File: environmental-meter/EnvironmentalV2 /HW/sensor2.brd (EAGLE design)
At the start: 66.7 x 50.6 mm, 16 parts

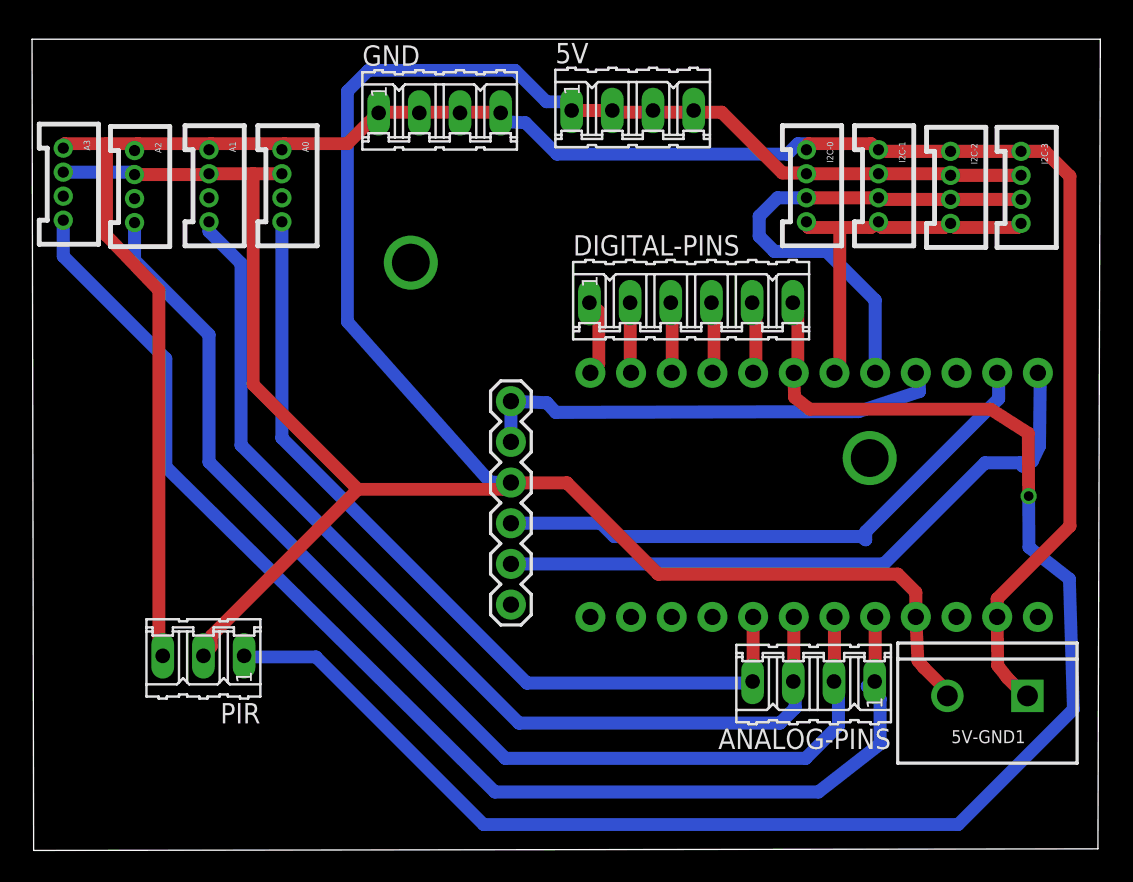
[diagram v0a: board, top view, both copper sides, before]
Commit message: EnvironmentalV2 update version
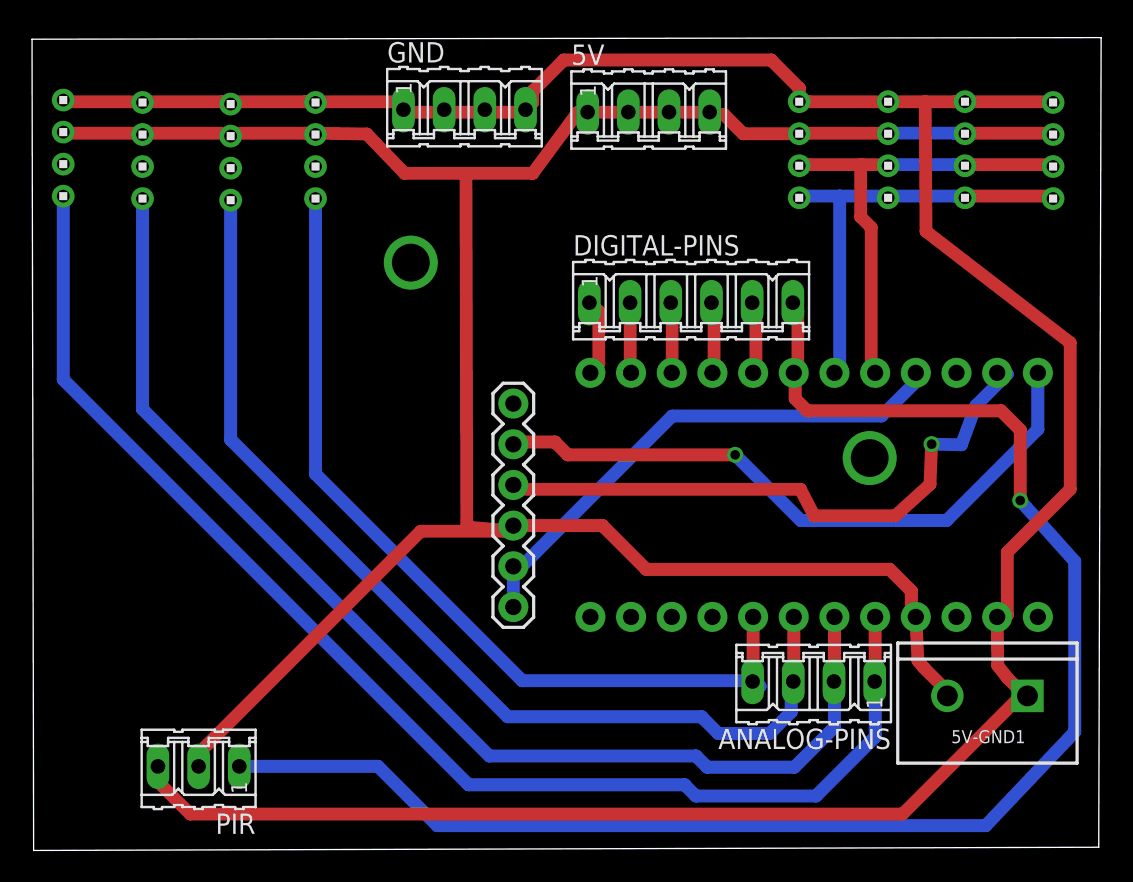
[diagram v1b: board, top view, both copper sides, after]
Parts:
- A0, A1, A2, A3, I2C-0, I2C-1, I2C-2, I2C-3: value (none) -> 1X4; device SparkFun-Connectors:1X04-1.5MM_JST -> headers(2mm):1X4
- moved JP3 12.6 mm to (58.1, 53.8), turned to 270 degrees
- moved PIR 6.91 mm to (38.5, 31.1)
- moved A0 2.10 mm to (45.8, 69.5)
- moved I2C-3 2.00 mm to (91.8, 69.5)
- moved GND 1.56 mm to (55.0, 72.1)
- moved A1 1.36 mm to (40.5, 69.5)
- moved 5V 1.00 mm to (66.5, 72.0)
- moved I2C-2 0.91 mm to (86.3, 69.6)
- moved I2C-1 0.60 mm to (81.5, 69.6)
- moved A2 0.50 mm to (35.0, 69.5)
- moved I2C-0 0.45 mm to (76.0, 69.6)
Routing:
- net GND: track 136.6 -> 169.5 mm
- net N$5: track 170.2 -> 150.9 mm
- net N$3: track 29.8 -> 33.6 mm
- net N$1: track 23.4 -> 27.2 mm
- net N$4: track 32.2 -> 29.3 mm
- net N$6: track 71.6 -> 73.5 mm
- net N$10: track 36.4 -> 38.4 mm, vias 0 -> 1
- net N$9: track 53.3 -> 55.1 mm
- net N$17: track 99.2 -> 97.7 mm
- net N$7: track 62.7 -> 64.1 mm
- net N$2: track 80.6 -> 82.0 mm
- net N$8: track 41.1 -> 40.7 mm, vias 0 -> 1
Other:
- board size 66.7 x 50.6 mm -> 66.8 x 50.7 mm
